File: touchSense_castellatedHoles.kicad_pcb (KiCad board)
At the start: 2 copper layers, 15 x 10 mm, 12 parts, among them J1 breakout, J2 GS2, U1 AT42QT1010-TSHR

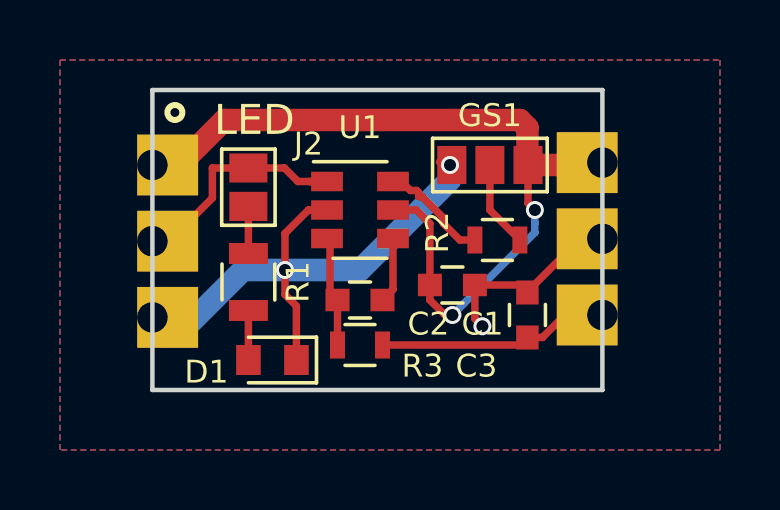
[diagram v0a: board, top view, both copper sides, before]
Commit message: organize project folder, small pcb maitenance, generated gerbers
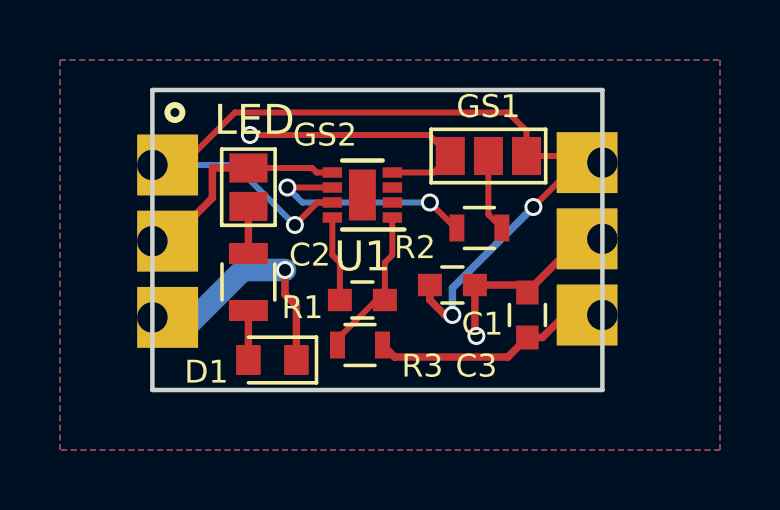
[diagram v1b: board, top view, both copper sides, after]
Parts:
- U1: value AT42QT1010-TSHR -> VDFN-8-1EP_2x2mm_Pitch0.5mm; footprint TO_SOT_Packages_SMD:SOT-23-6 -> Housings_DFN_QFN:VDFN-8-1EP_2x2mm_Pitch0.5mm
- moved R2 0.72 mm to (116.0, 104.6)
- moved U1 0.51 mm to (112.1, 103.5), turned to 180 degrees
- moved GS1 0.30 mm to (116.3, 102.2)
- moved C2 0.08 mm to (112.1, 107.0), turned to 180 degrees
- renumbered J2 to GS2
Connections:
- U1 pad 1: /OUT1 -> Net-(C2-Pad1)
- U1 pad 2: GND -> (no net)
- U1 pad 3: Net-(C2-Pad1) -> (no net)
- U1 pad 4: Net-(C2-Pad2) -> GND
- U1 pad 5: /VDD -> /OUT1
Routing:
- net /VDD: track 28.8 -> 35.1 mm, vias 2 -> 3
- net Net-(R2-Pad2): track 3.73 -> 7.86 mm, vias 0 -> 2
- net /OUT1: track 10.4 -> 8.08 mm
- net Net-(C2-Pad1): track 3.69 -> 5.17 mm
- net GND: track 25.4 -> 24.2 mm
- net Net-(C2-Pad2): track 2.19 -> 2.85 mm
